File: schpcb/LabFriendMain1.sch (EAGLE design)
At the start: 654 parts, among them IC1 TPS62240DDC, IC10 TPS62240DDC, IC11 TPS73001DBVR, IC12 TPS73001DBVR, IC13 AK4621, IC14 TPS72301, IC15 LME49721, IC16 NE5532, IC17 OPA2134, IC18 LM8272, IC19 LMV358MM, IC2 25px80, IC20 ISL54405IRTZ, IC21 NE5532, IC22 74HC4052D, IC23 LME49721, IC24 74HC00D, IC25 INA331IDGK, IC26 MT41J128M8, IC27 74HCT132D, IC28 TPS72301, IC29 TPS73001DBVR, IC3 SI8462, IC30 LM8272, IC31 LMV358MM, IC32 ADS1118IDGSR, IC33 ADA4853-3RU, IC34 4052D, IC35 4052D, IC36 OPA2354, IC37 74HC595D, IC38 ADA4853-3RU, IC39 4052D, IC4 FT232H, IC40 4052D, IC41 OPA2354, IC42 74HC595D, IC43 LM321MF, IC44 74HC595D, IC5 ADC08200, IC6 ADC08200, IC7 TPS73001DBVR, IC8 93LC56SM, IC9 74LVC8T245, K1 G6K-2F-Y, K2 G6K-2F-Y, K3 G6K-2F-Y, K4 G6K-2F-Y, Q1 12MHz, Q2 FDN335N, Q3 FDN335N, T1 EFD15DCDCPM5P33EFD15, T10 BC850, T11 BC850, T12 BC856ASMD, T13 BC856ASMD, T14 BC850, T15 BC856ASMD, T16 BC850, T17 BC856ASMD, T2 BC850, T3 BC850, T4 BC850, T5 BC856ASMD, T6 BC856ASMD, T7 BC856ASMD, T8 BC850, T9 BC856ASMD, U2 6SLX9FTG256, X1 MINI-USB-32005-201, X2 31-5431-10RFX, X3 31-5431-10RFX

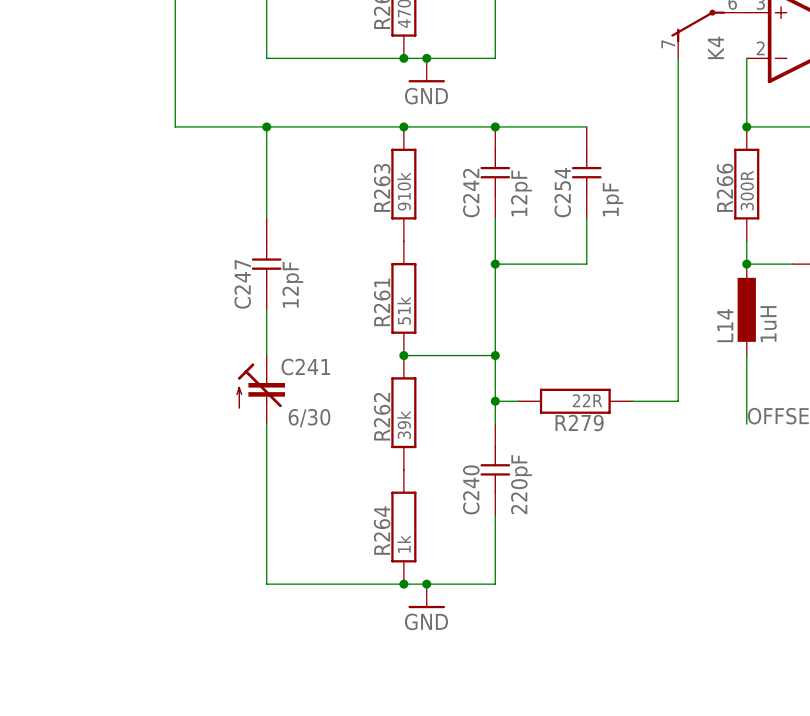
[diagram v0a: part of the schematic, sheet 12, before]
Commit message: many improovments and bugfixes and added features
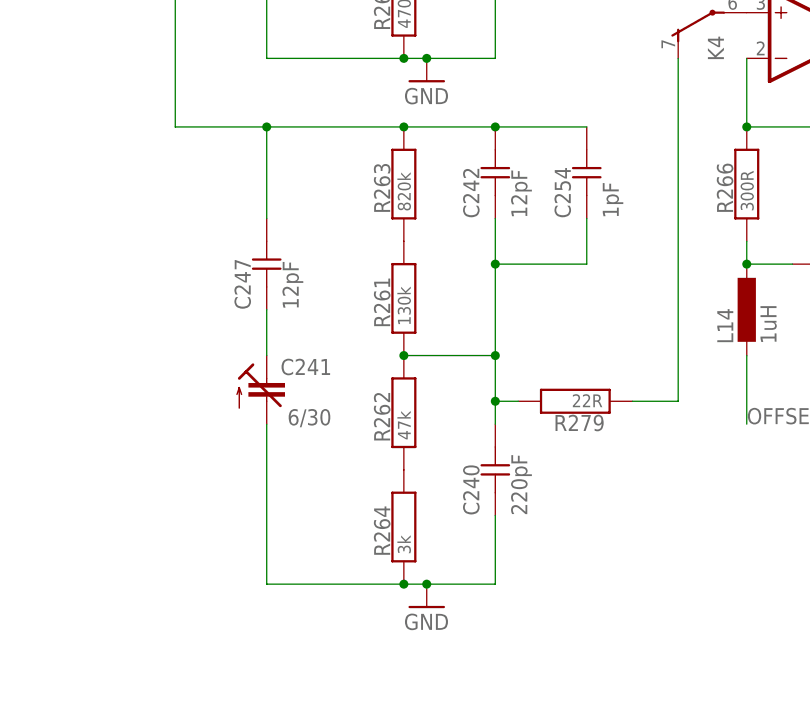
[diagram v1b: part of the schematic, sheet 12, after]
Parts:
- R261: value 51k -> 130k
- R262: value 39k -> 47k
- R263: value 910k -> 820k
- R264: value 1k -> 3k
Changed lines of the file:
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@@
 <?xml version="1.0" encoding="utf-8"?>
 <!DOCTYPE eagle SYSTEM "eagle.dtd">
-<eagle version="7.2.0">
+<eagle version="7.7.0">
 <drawing>
 <settings>
@@
 <part name="R260" library="passive" deviceset="RES" device="R0603" value="470k"/>
 <part name="C239" library="passive" deviceset="CAP" device="C0603" value="12pF"/>
-<part name="R261" library="passive" deviceset="RES" device="R0603" value="51k"/>
+<part name="R261" library="passive" deviceset="RES" device="R0603" value="130k"/>
 <part name="C240" library="passive" deviceset="CAP" device="C0603" value="220pF"/>
-<part name="R262" library="passive" deviceset="RES" device="R0603" value="39k"/>
+<part name="R262" library="passive" deviceset="RES" device="R0603" value="47k"/>
 <part name="GND151" library="supply1" deviceset="GND" device=""/>
 <part name="C241" library="rcl" deviceset="C-TRIMM" device="TZBX4" value="6/30"/>
-<part name="R263" library="passive" deviceset="RES" device="R0603" value="910k"/>
-<part name="R264" library="passive" deviceset="RES" device="R0603" value="1k"/>
+<part name="R263" library="passive" deviceset="RES" device="R0603" value="820k"/>
+<part name="R264" library="passive" deviceset="RES" device="R0603" value="3k"/>
 <part name="C242" library="passive" deviceset="CAP" device="C0603" value="12pF"/>
 <part name="R265" library="passive" deviceset="RES" device="R0603" value="300R"/>
@@
 <pinref part="C187" gate="G$1" pin="2"/>
 <junction x="81.28" y="40.64"/>
-<pinref part="C187" gate="G$1" pin="2"/>
 </segment>
 <segment>
@@
 <pinref part="C186" gate="G$1" pin="2"/>
 <junction x="170.18" y="68.58"/>
-<pinref part="C186" gate="G$1" pin="2"/>
 </segment>
 <segment>
